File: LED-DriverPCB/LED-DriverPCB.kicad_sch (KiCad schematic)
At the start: 53 parts, among them J1 Screw_Terminal_01x03, J12 Screw_Terminal_01x02, J13 Screw_Terminal_01x02, J14 Screw_Terminal_01x02, J15 Screw_Terminal_01x02, J16 Screw_Terminal_01x02, J17 Screw_Terminal_01x02, J18 Screw_Terminal_01x02, J19 Screw_Terminal_01x02, J2 Screw_Terminal_01x03, J20 Conn_ARM_SWD_TagConnect_TC2030, J3 Screw_Terminal_01x03, J4 Screw_Terminal_01x03, J5 Screw_Terminal_01x03, J6 Screw_Terminal_01x03, J7 Screw_Terminal_01x03, J8 Screw_Terminal_01x03, J9 USB_C_Receptacle_USB2.0_16P, U1 STM32F103RCTx, U2 TXB0108PW, U3 AMS1117-3.3, U4 USBLC6-2SC6, X1 8MHz

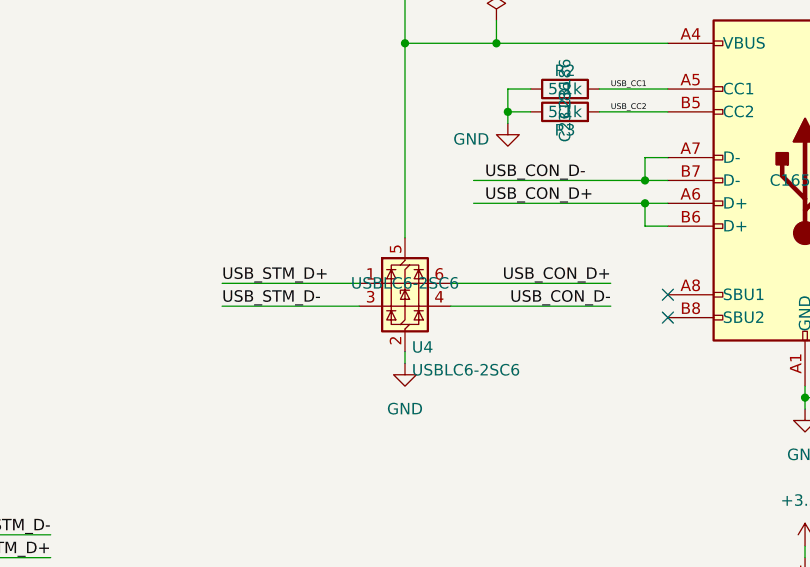
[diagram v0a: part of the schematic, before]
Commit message: Created manufaturing files
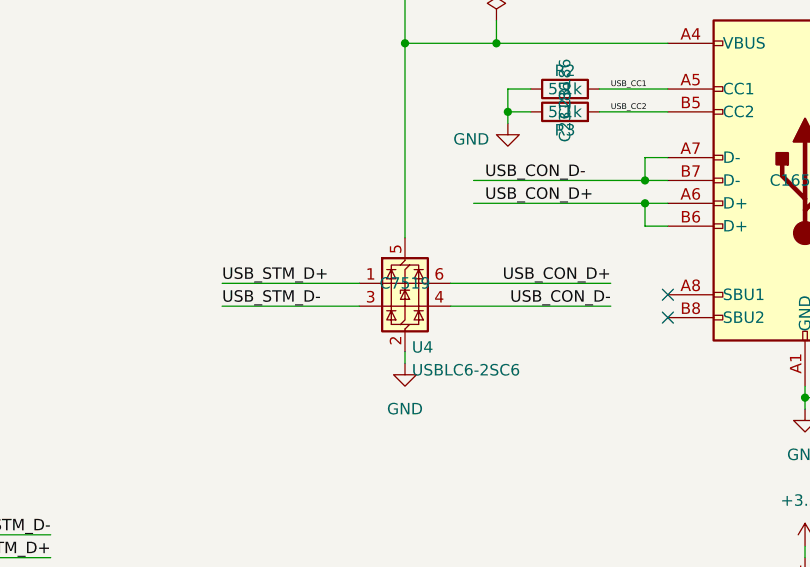
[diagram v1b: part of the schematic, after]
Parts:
- U4: JLCPCB Part # USBLC6-2SC6 -> C7519
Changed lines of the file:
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@@
 			)
 		)
-		(property "JLCPCB Part #" "USBLC6-2SC6"
+		(property "JLCPCB Part #" "C7519"
 			(at 189.23 69.85 0)
 			(effects
